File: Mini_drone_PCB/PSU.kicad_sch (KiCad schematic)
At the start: 15 parts, among them J1 Power IN, U1 TPS62085RLTR, U2 470nH 6.9mΩ, U6 INA236AIDDFR

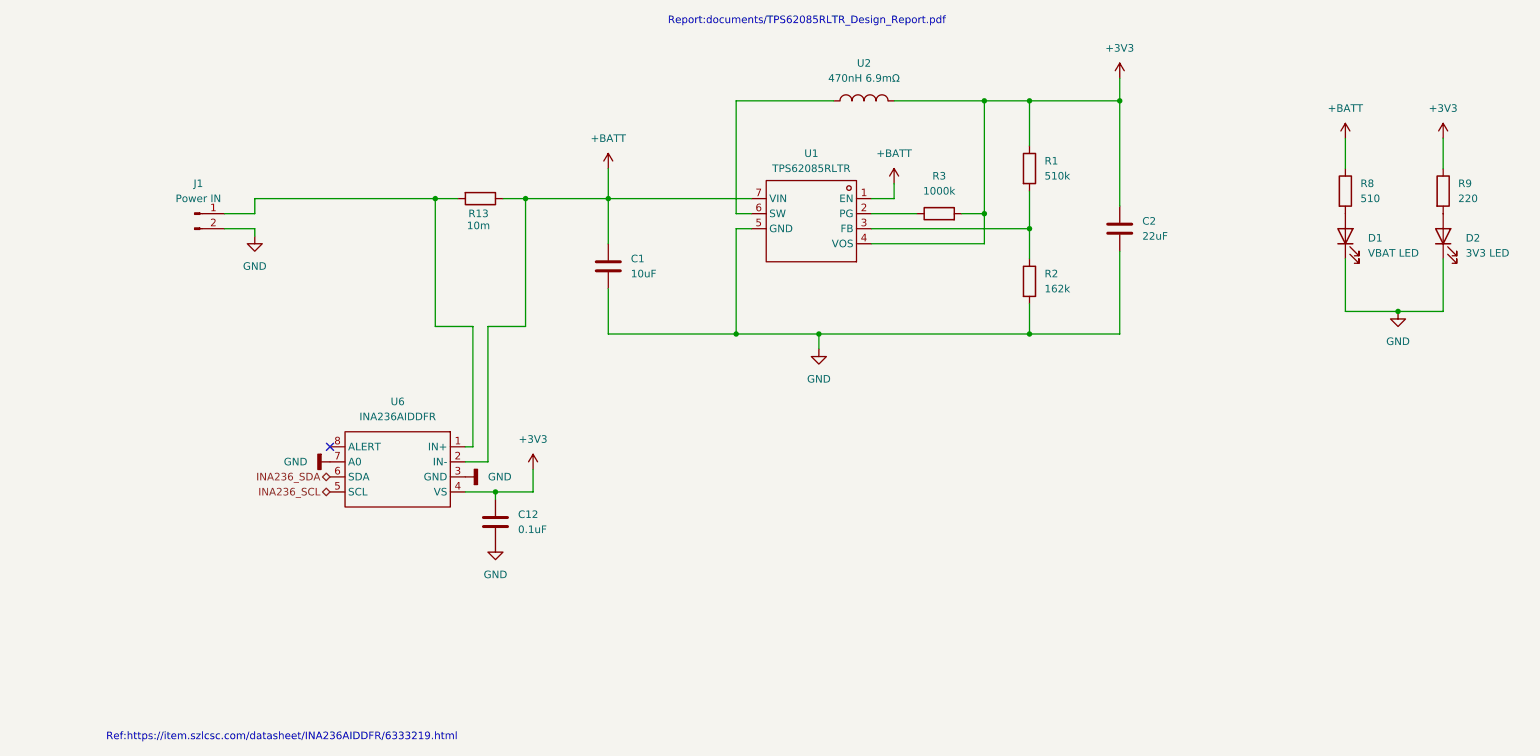
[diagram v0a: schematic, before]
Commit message: fix sch
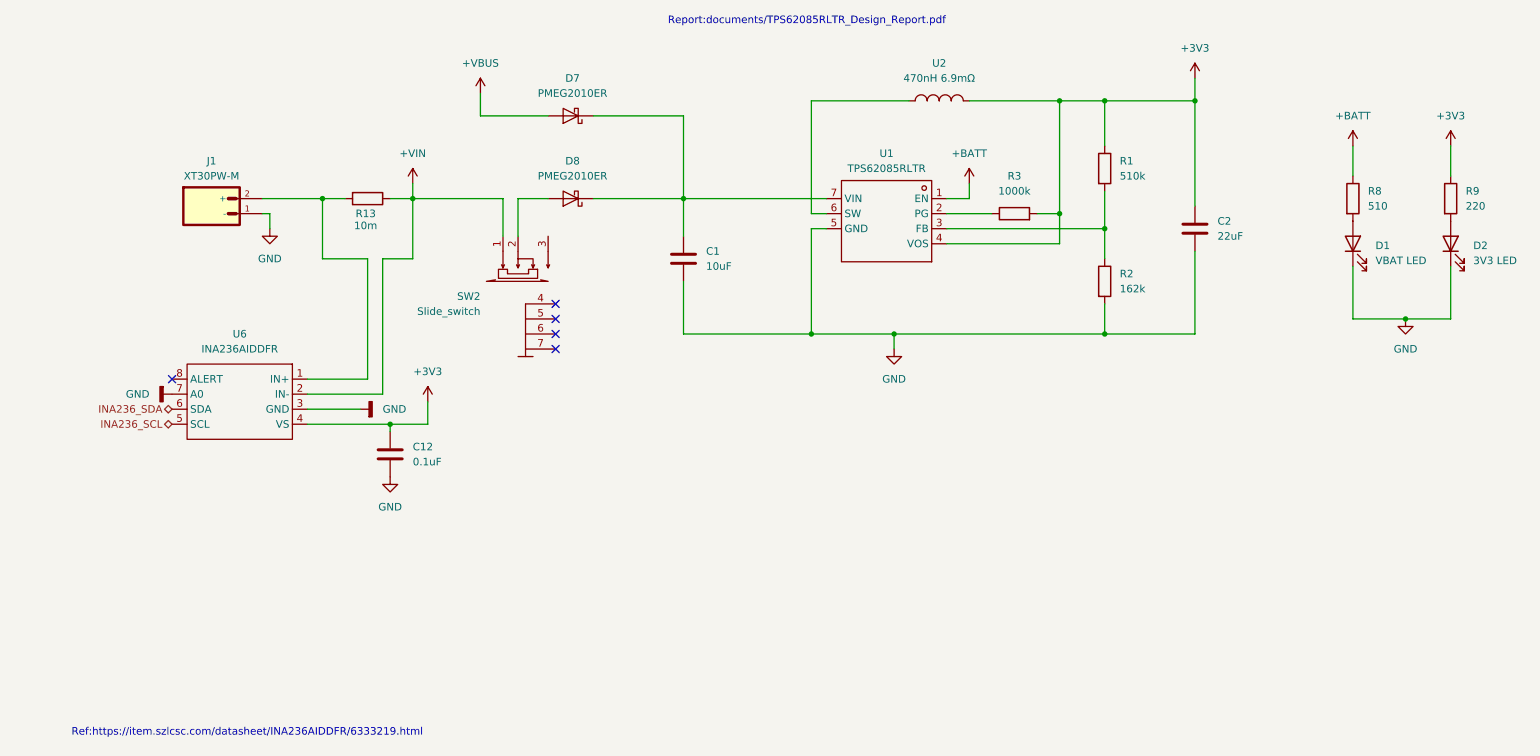
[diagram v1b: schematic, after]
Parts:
- removed J1: Power IN, Connector_JST:JST_PH_S2B-PH-K_1x02_P2.00mm_Horizontal, symbol Connector:Conn_01x02_Pin
- added D7, D8: PMEG2010ER, Diode_SMD:Nexperia_CFP3_SOD-123W, symbol Diode:PMEG2010ER
- added J1: XT30PW-M, Sharing_Footprint:AMASS_XT30PW-M, symbol Sharing_Symbol:XT30PW-M
- added SW2: Slide_switch, mini_drone:SW-SMD_SSSS811101, symbol mini_drone:SSSS811101
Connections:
- net +BATT: no longer C1.1, R13.1, U1.7 (VIN), U6.2 (IN-)
- net GND: now also J1.1 (-)
- net at R13.2, U6.1 (IN+): now also J1.2 (+)
- new net: C1.1, D7.1 (K), D8.1 (K), U1.7 (VIN)
- new net: D8.2 (A), SW2.2
- new net +VBUS: D7.2 (A)
- new net +VIN: R13.1, SW2.1, U6.2 (IN-)
- no-connect marks 1 -> 5
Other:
- moved on the sheet: C1, C12, C2, D1, D2, R1, R13, R2, R3, R8, R9, U1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
